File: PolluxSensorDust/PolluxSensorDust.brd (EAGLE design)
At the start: 26.3 x 25.4 mm, 5 parts

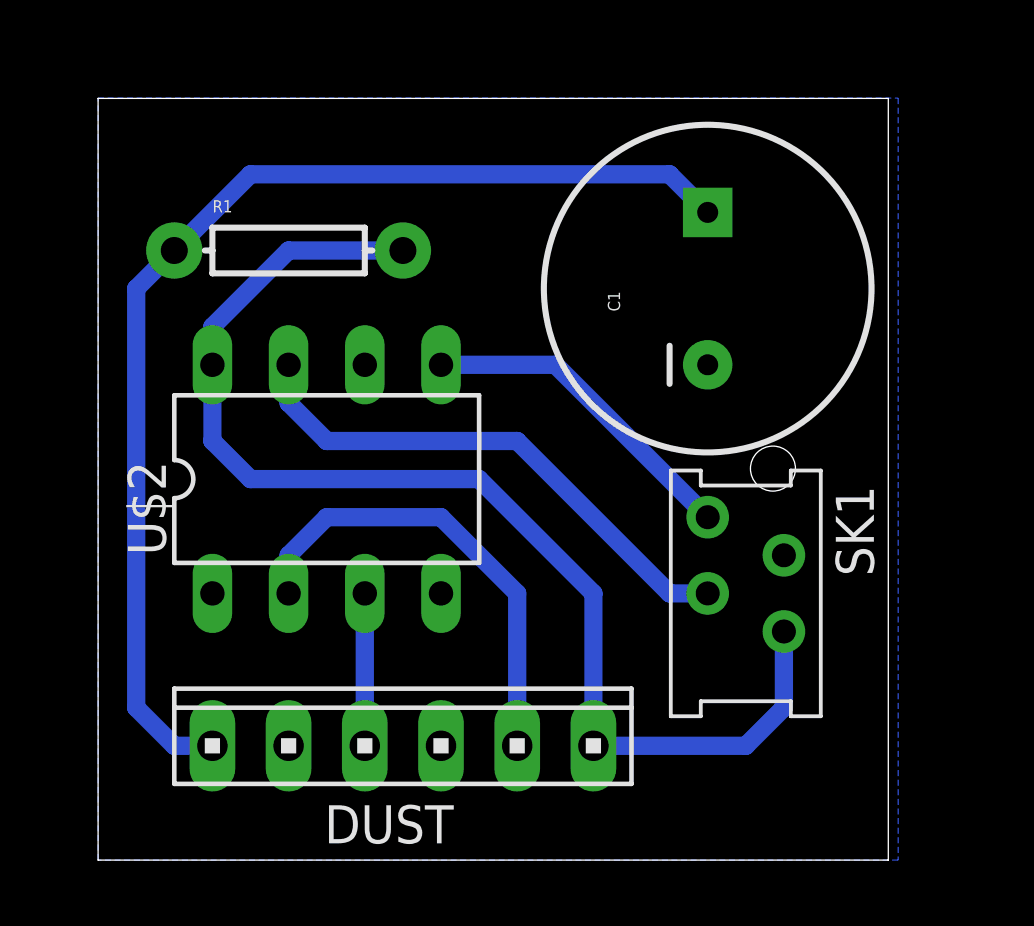
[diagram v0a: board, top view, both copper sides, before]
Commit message: improve sensor board
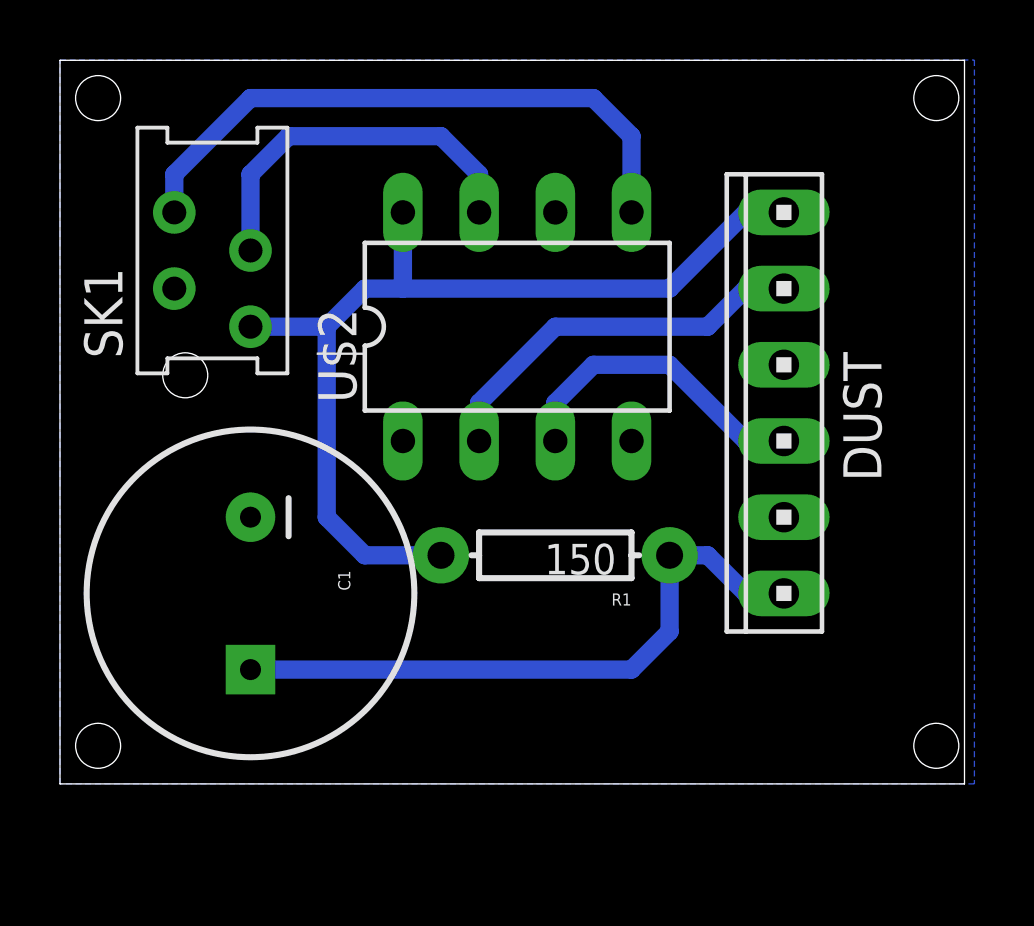
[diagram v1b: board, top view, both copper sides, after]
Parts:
- C1: value (none) -> 220 uF
- R1: value (none) -> 150
- moved SK1 18.9 mm to (15.2, 24.1), turned to 90 degrees
- moved C1 18.3 mm to (16.5, 15.2), turned to 270 degrees
- moved DUST 17.1 mm to (34.3, 21.6), turned to 90 degrees
- moved R1 13.5 mm to (26.7, 16.5), turned to 180 degrees
- moved U$2 8.13 mm to (25.4, 24.1)
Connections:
- removed net N$2: SK1.1, U$2.5
- new net SDA: SK1.4, U$2.5
- net 5V: now also SK1.1; no longer SK1.4
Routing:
- net SDA: track 0.00 -> 20.6 mm
- net N$4: track 38.2 -> 21.4 mm
- net N$2: track 11.0 -> 0.00 mm
- net 5V: track 40.5 -> 32.6 mm
- net N$1: track 17.9 -> 12.5 mm
- net DUST_LED: track 5.08 -> 10.5 mm
- net DUST_READ: track 15.5 -> 13.0 mm
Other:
- board size 26.3 x 25.4 mm -> 30.2 x 24.1 mm
